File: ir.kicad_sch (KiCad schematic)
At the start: 38 parts

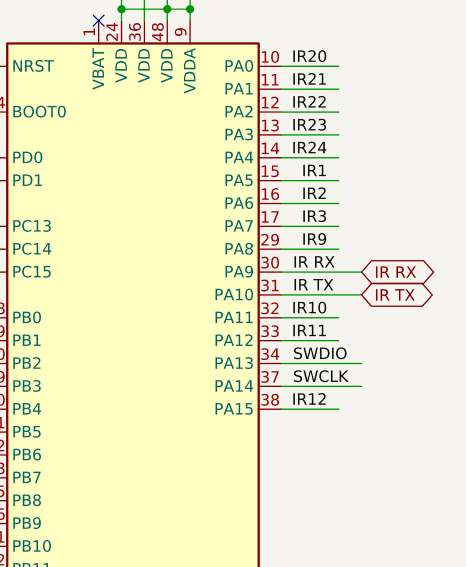
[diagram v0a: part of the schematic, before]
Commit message: i wanna kill myself
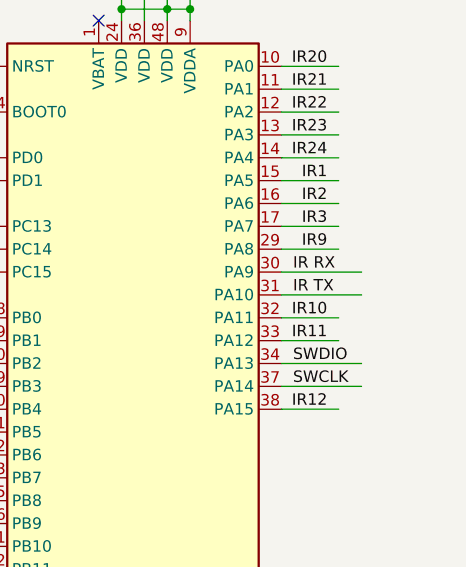
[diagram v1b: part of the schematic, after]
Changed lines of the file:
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@@
     (effects (font (size 1.27 1.27)) (justify right bottom))
-  )
-  (global_label "IR RX" (shape bidirectional) (at 274.32 85.09 0)
-    (effects (font (size 1.27 1.27)) (justify left))
-    (property "Intersheetrefs" "${INTERSHEET_REFS}" (at 282.2141 85.09 0)
-      (effects (font (size 1.27 1.27)) hide)
-    )
-  )
-  (global_label "IR TX" (shape bidirectional) (at 274.32 87.63 0)
-    (effects (font (size 1.27 1.27)) (justify left))
-    (property "Intersheetrefs" "${INTERSHEET_REFS}" (at 282.2141 87.63 0)
-      (effects (font (size 1.27 1.27)) hide)
-    )
   )
   (symbol (lib_id "Device:C") (at 204.47 69.85 270) (unit 1)
